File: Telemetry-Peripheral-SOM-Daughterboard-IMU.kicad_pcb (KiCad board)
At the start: 2 copper layers, 24 x 50 mm, 17 parts, among them IC1 LMT87LPG, IC2 FS3000-1015, J1 Conn_02x10_Odd_Even, U1 LSM6DSV, U2 LSM6DSV

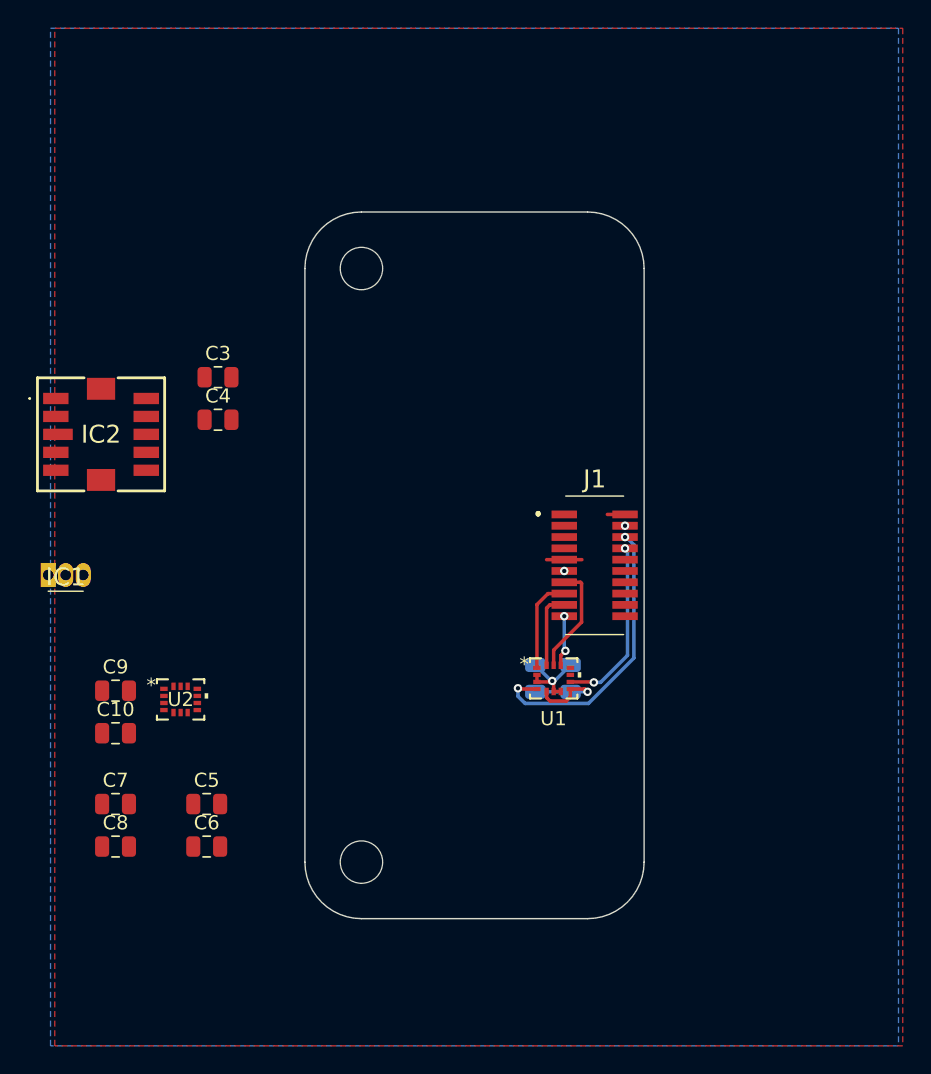
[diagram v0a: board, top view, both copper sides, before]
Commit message: first draft
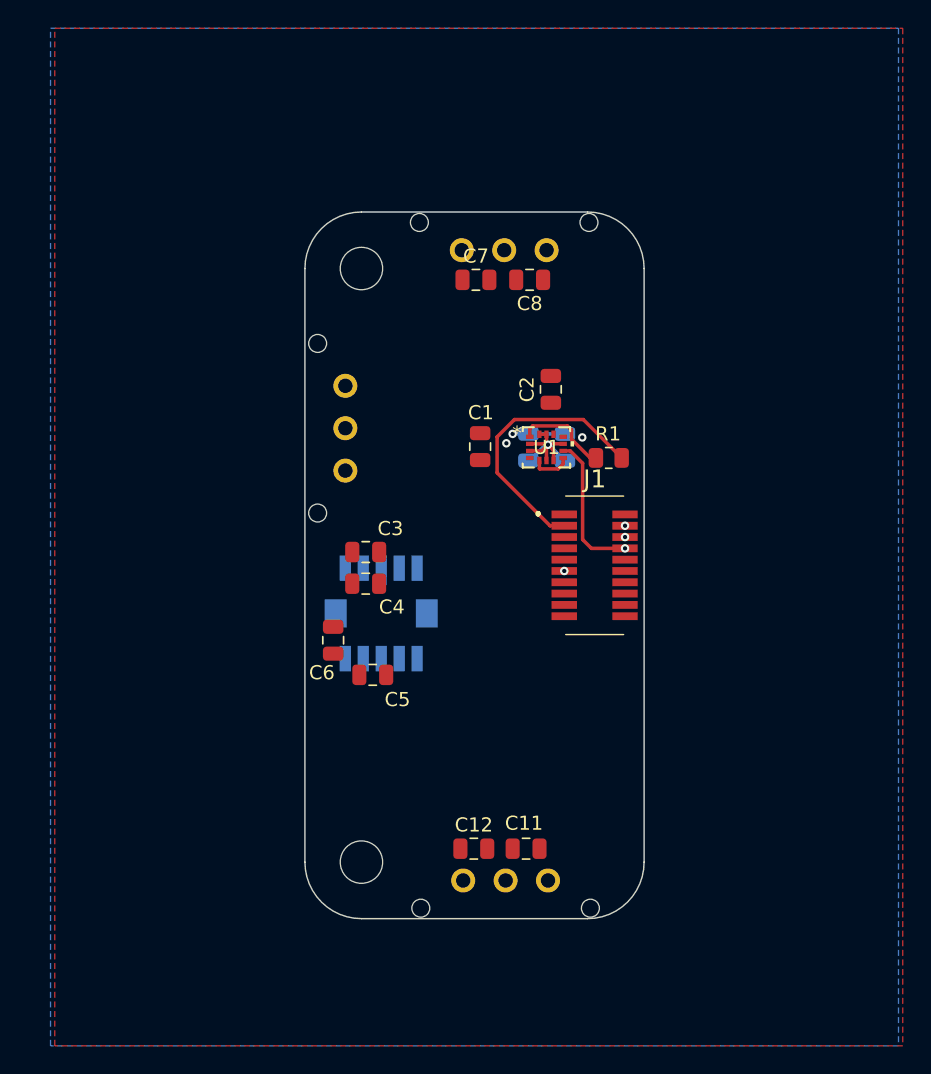
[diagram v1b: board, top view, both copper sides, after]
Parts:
- removed IC2: FS3000-1015, UTSVT_Special:FS30001015
- removed U2: LSM6DSV, UTSVT_Special:LGA14-L_2P59X3P1X0P5_STM
- added C11: 10n, Capacitor_SMD:C_0805_2012Metric, F.Cu at (161.7, 111.0)
- added C12: 0.1u, Capacitor_SMD:C_0805_2012Metric, F.Cu at (157.9, 111.0)
- added J2: Conn_01x03_Pin, UTSVT_Connectors:Molex_MicroFit3.0_1x3xP3.00mm_PolarizingPeg_Vertical, B.Cu at (163.1, 68.7)
- added J3: Conn_01x03_Pin, UTSVT_Connectors:Molex_MicroFit3.0_1x3xP3.00mm_PolarizingPeg_Vertical, B.Cu at (148.9, 78.3)
- added J4: Conn_01x03_Pin, UTSVT_Connectors:Molex_MicroFit3.0_1x3xP3.00mm_PolarizingPeg_Vertical, B.Cu at (157.2, 113.3)
- added R1: 50, Resistor_SMD:R_0805_2012Metric, F.Cu at (167.5, 83.4)
- C1, C2: moved to F.Cu
- C10: moved to B.Cu
- C7: value 0.1u -> 10n
- C9: value 0.1u -> 10n; moved to B.Cu
- IC1: value LMT87LPG -> FS3000-1015; footprint UTSVT_ICs:LMT87LPG -> UTSVT_Special:FS30001015; moved to B.Cu
- U1: footprint UTSVT_ICs:LGA14-L_2P59X3P1X0P5_STM -> UTSVT_Special:LGA14-L_2P59X3P1X0P5_STM
- moved C8 49.7 mm to (161.9, 70.8), turned to 180 degrees
- moved C7 45.0 mm to (158.1, 70.8)
- moved C10 37.7 mm to (164.4, 82.7), turned to -90 degrees
- moved C9 33.9 mm to (161.8, 82.6), turned to -90 degrees
- moved IC1 23.7 mm to (151.4, 94.4), turned to -90 degrees
- moved C2 20.5 mm to (163.4, 78.5)
- moved C6 17.1 mm to (148.0, 96.3), turned to -90 degrees
- moved C1 16.9 mm to (158.4, 82.6), turned to -90 degrees
- moved U1 16.4 mm to (163.1, 82.7)
- moved C3 16.2 mm to (150.3, 90.1)
- moved C4 15.6 mm to (150.3, 92.3)
- moved C5 14.9 mm to (150.8, 98.8), turned to 180 degrees
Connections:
- C4 pad 1: Net-(IC2-VREG) -> Net-(IC1-VREG)
- C5 pad 1: Net-(IC2-TP1) -> Net-(IC1-TP1)
- C5 pad 2: Net-(IC2-TP2) -> Net-(IC1-TP2)
- C6 pad 1: Net-(IC2-VCM) -> Net-(IC1-VCM)
- C9 pad 1: +3.3V -> /ADC1_IN
- IC1 pad 1: /SPI1_NSS -> Net-(IC1-VREG)
- IC1 pad 2: GND -> +3.3V
- IC1 pad 3: +3.3V -> GND
- J1 pad 2: +3.3V -> /ADC1_IN
- J1 pad 4: GND -> /ADC2_IN
- U1 pad 1: /SPI1_MISO -> Net-(U1-SDO/SA0)
- U1 pad 12: /SPI1_NSS -> /SPI2_NSS
- U1 pad 13: /SPI1_SCK -> /SPI2_SCK
- U1 pad 14: /SPI1_MOSI -> /SPI2_MOSI
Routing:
- net /I2C2_SDA: track 20.5 -> 0.15 mm
- net /SPI2_MISO: track 0.00 -> 19.3 mm
- net /SPI1_SCK: track 7.87 -> 0.00 mm
- net /SPI1_MISO: track 6.72 -> 0.00 mm
- net Net-(U1-SDO/SA0): track 0.00 -> 6.65 mm
- net /SPI1_MOSI: track 5.39 -> 0.00 mm
- net +3.3V: track 11.6 -> 6.53 mm
- net GND: track 6.33 -> 11.1 mm, vias 3 -> 2
- net /SPI1_NSS: track 3.64 -> 0.00 mm, vias 2 -> 0
- net /I2C2_SCL: track 12.5 -> 10.4 mm
- net /ADC2_IN: vias 0 -> 1
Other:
- board text added: "Telemetry Peripheral SOM Daughterboard IMU Fall 2023 - Design by Andrew Nguyen, Frank Li, Jim Fang"
- board text removed: "Telemetry Peripheral SOM Daughterboard IMU Fall 2023 - Design by Andrew Nguyen"

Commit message: a
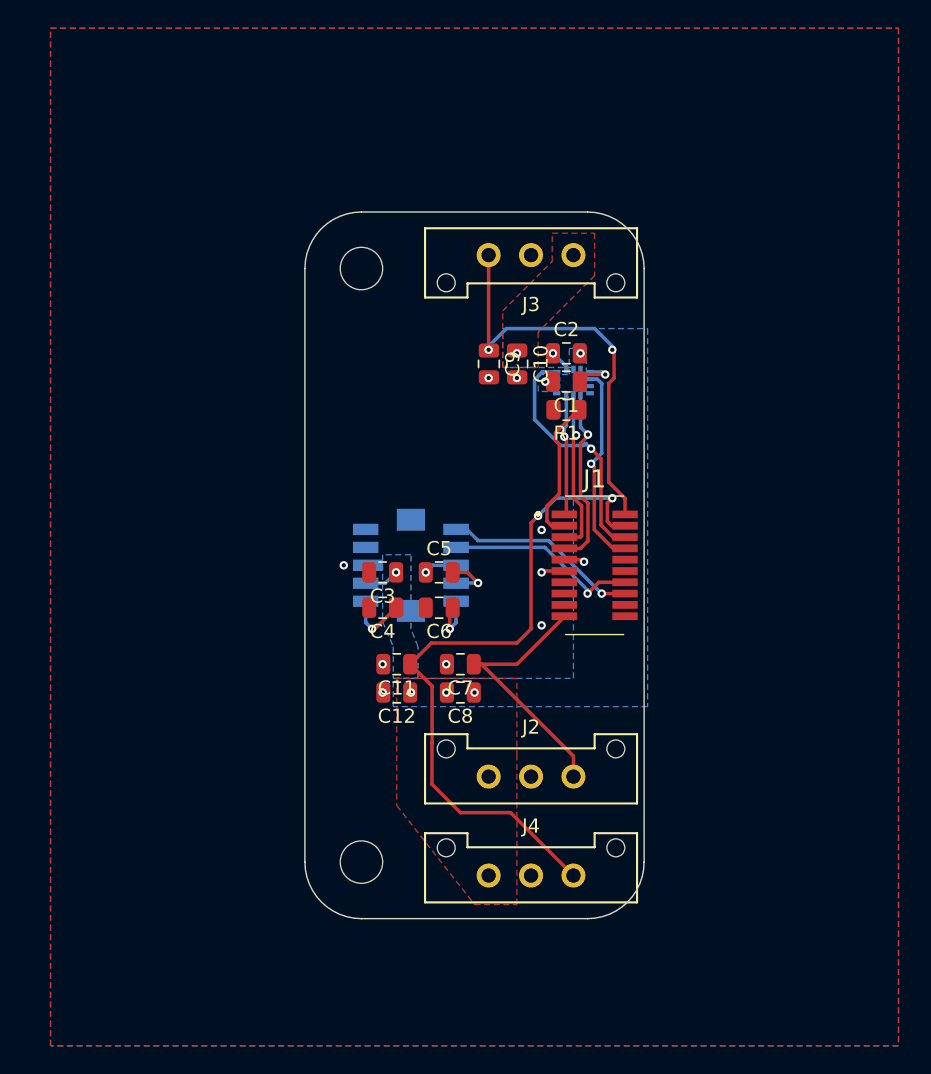
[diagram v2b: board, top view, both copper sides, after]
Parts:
- C10, C9, J2, J3, J4: moved to F.Cu
- U1: moved to B.Cu
- moved J2 37.5 mm to (159.0, 106.0), turned to 0 degrees
- moved C8 29.6 mm to (157.0, 100.0)
- moved C7 27.2 mm to (157.0, 98.0), turned to 180 degrees
- moved J3 18.6 mm to (165.0, 69.0), turned to 180 degrees
- moved C11 15.9 mm to (152.5, 98.0)
- moved C12 12.3 mm to (152.5, 100.0), turned to 180 degrees
- moved C5 8.64 mm to (155.5, 91.5), turned to 0 degrees
- moved C6 7.84 mm to (155.5, 94.0), turned to 180 degrees
- moved C1 7.64 mm to (164.5, 78.0), turned to 180 degrees
- moved C10 6.80 mm to (161.0, 76.8)
- moved C9 6.52 mm to (159.0, 76.8)
- moved U1 4.96 mm to (165.0, 78.1)
- moved R1 4.53 mm to (164.5, 80.0)
- moved IC1 4.00 mm to (153.5, 91.0), turned to 0 degrees
- moved C2 2.78 mm to (164.5, 76.0), turned to 0 degrees
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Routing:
- net /ADC2_IN: track 0.00 -> 48.6 mm, vias 1 -> 2
- net /ADC1_IN: track 0.00 -> 29.4 mm, vias 0 -> 2
- net /SPI1_NSS: track 0.00 -> 19.0 mm
- net /I2C2_SDA: track 0.15 -> 17.3 mm, vias 2 -> 1
- net /I2C1_SDA: track 0.00 -> 13.8 mm, vias 0 -> 1
- net /I2C1_SCL: track 0.00 -> 13.8 mm, vias 0 -> 1
- net /SPI2_NSS: track 0.00 -> 12.8 mm, vias 0 -> 1
- net /SPI2_SCK: track 0.00 -> 11.6 mm, vias 0 -> 1
- net GND: track 11.1 -> 1.64 mm, vias 2 -> 12
- net /SPI2_MISO: track 19.3 -> 10.4 mm
- net /SPI2_MOSI: track 0.00 -> 8.59 mm, vias 0 -> 1
- net Net-(U1-SDO/SA0): track 6.65 -> 0.00 mm
- net Net-(IC1-VREG): track 0.00 -> 4.47 mm, vias 0 -> 1
- net /I2C2_SCL: track 10.4 -> 14.4 mm, vias 2 -> 1
- net Net-(IC1-VCM): track 0.00 -> 3.73 mm, vias 0 -> 1
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- added copper zone on B.Cu, net +3.3V
- added copper zone on F.Cu, net GND
